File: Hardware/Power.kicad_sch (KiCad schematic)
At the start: 13 parts, among them U22 TLV75733PDRV, U7 SY8205FCC, U9 AP2112K-1.8

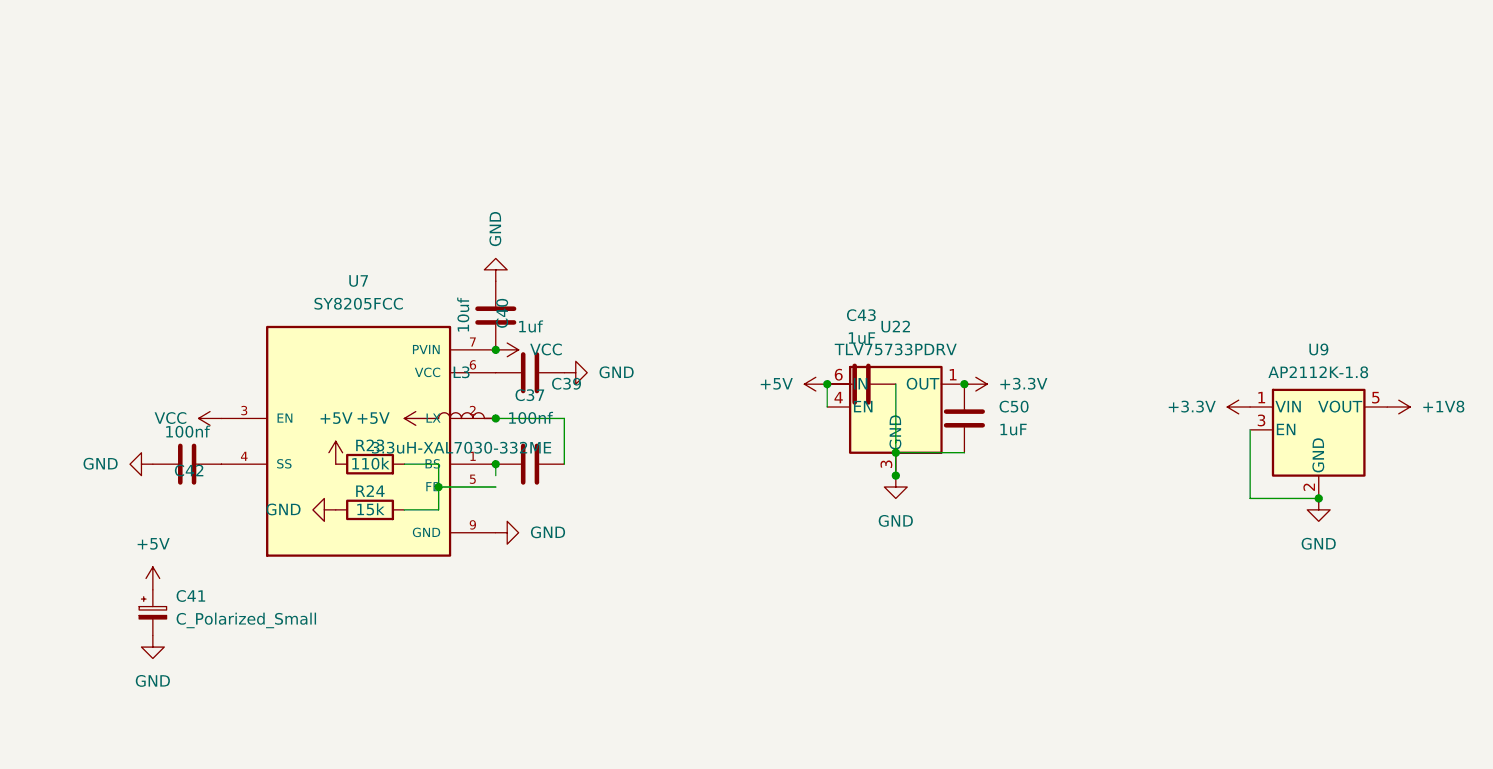
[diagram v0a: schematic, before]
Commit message: 12-March update
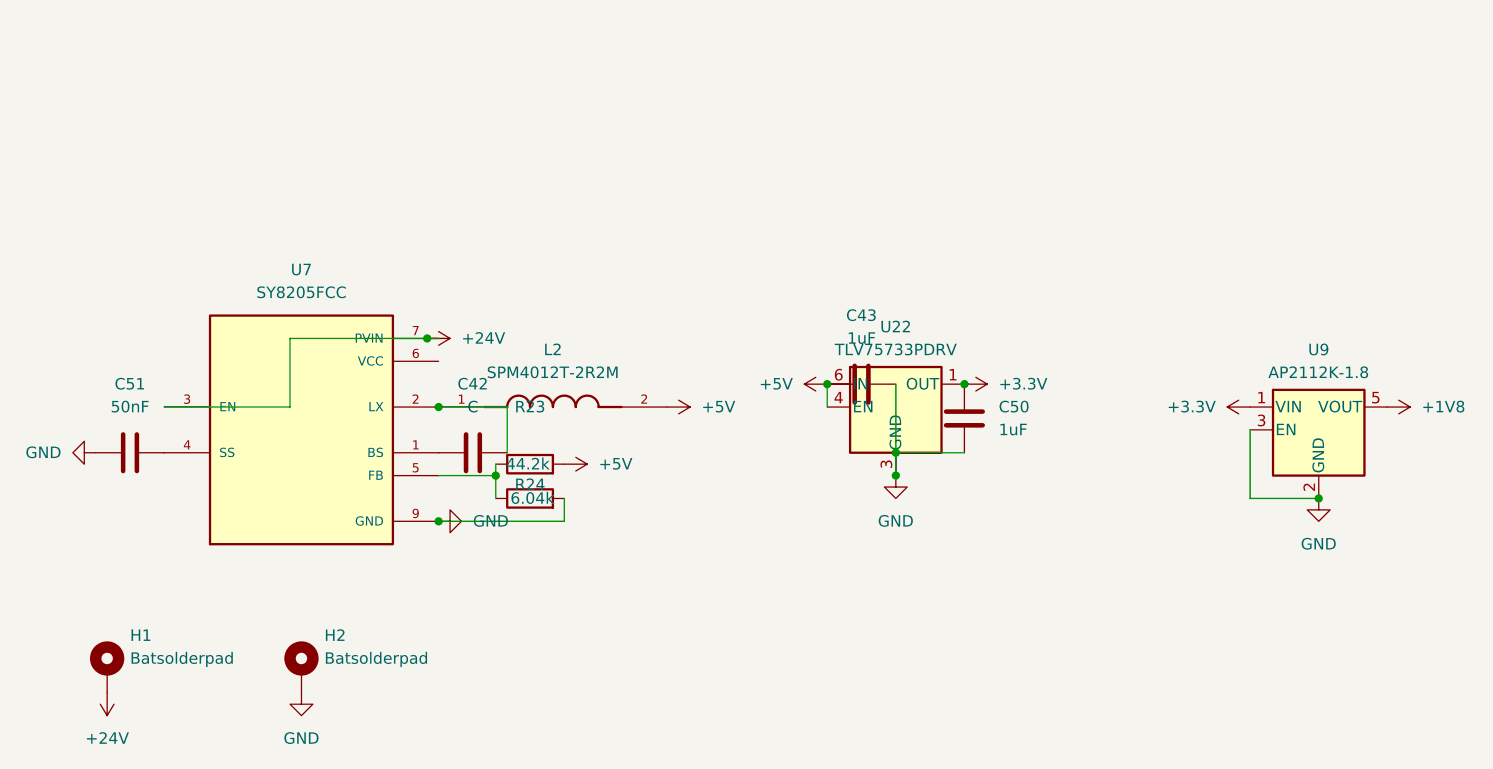
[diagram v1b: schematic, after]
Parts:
- removed C37: 100nf, Capacitor_SMD:C_1206_3216Metric_Pad1.33x1.80mm_HandSolder, symbol Device:C
- removed C39: 1uf, Capacitor_SMD:C_1206_3216Metric_Pad1.33x1.80mm_HandSolder, symbol Device:C
- removed C40: 10uf, Capacitor_SMD:C_0402_1005Metric, symbol Device:C
- removed C41: C_Polarized_Small, Capacitor_SMD:CP_Elec_3x5.3, symbol Device:C_Polarized_Small
- removed L3: 3.3uH-XAL7030-332ME, Inductor_SMD:L_6.3x6.3_H3, symbol Device:L
- added C51: 50nF, Capacitor_SMD:C_0201_0603Metric, symbol Device:C
- added H1, H2: Batsolderpad, TestPoint:TestPoint_Pad_4.0x4.0mm, symbol Mechanical:Batsolderpad
- added L2: SPM4012T-2R2M, SPM4012T-2R2M:IND_SPM4012T-2R2M, symbol SPM4012T-2R2M:SPM4012T-2R2M
- C42: value 100nf -> C; footprint Capacitor_SMD:C_0402_1005Metric -> (none)
- R23: value 110k -> 44.2k; footprint Resistor_SMD:R_0508_1220Metric_Pad1.12x2.15mm_HandSolder -> Resistor_SMD:R_0402_1005Metric
- R24: value 15k -> 6.04k; footprint Resistor_SMD:R_0508_1220Metric -> Resistor_SMD:R_0402_1005Metric
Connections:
- net +5V: now also R23.2, L2.2; no longer R23.1
- net GND: now also R24.2, C51.1, H2.1; no longer C42.1, R24.1
- net at C42.2: now also U7.2 (LX), L2.1; no longer U7.4 (SS)
- net at U7.1 (BS): now also C42.1
- net PVIN renamed +24V
- net +24V: now also H1.1
- new net: R23.1, R24.1, U7.5 (FB)
- new net: C51.2, U7.4 (SS)

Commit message: test gpg
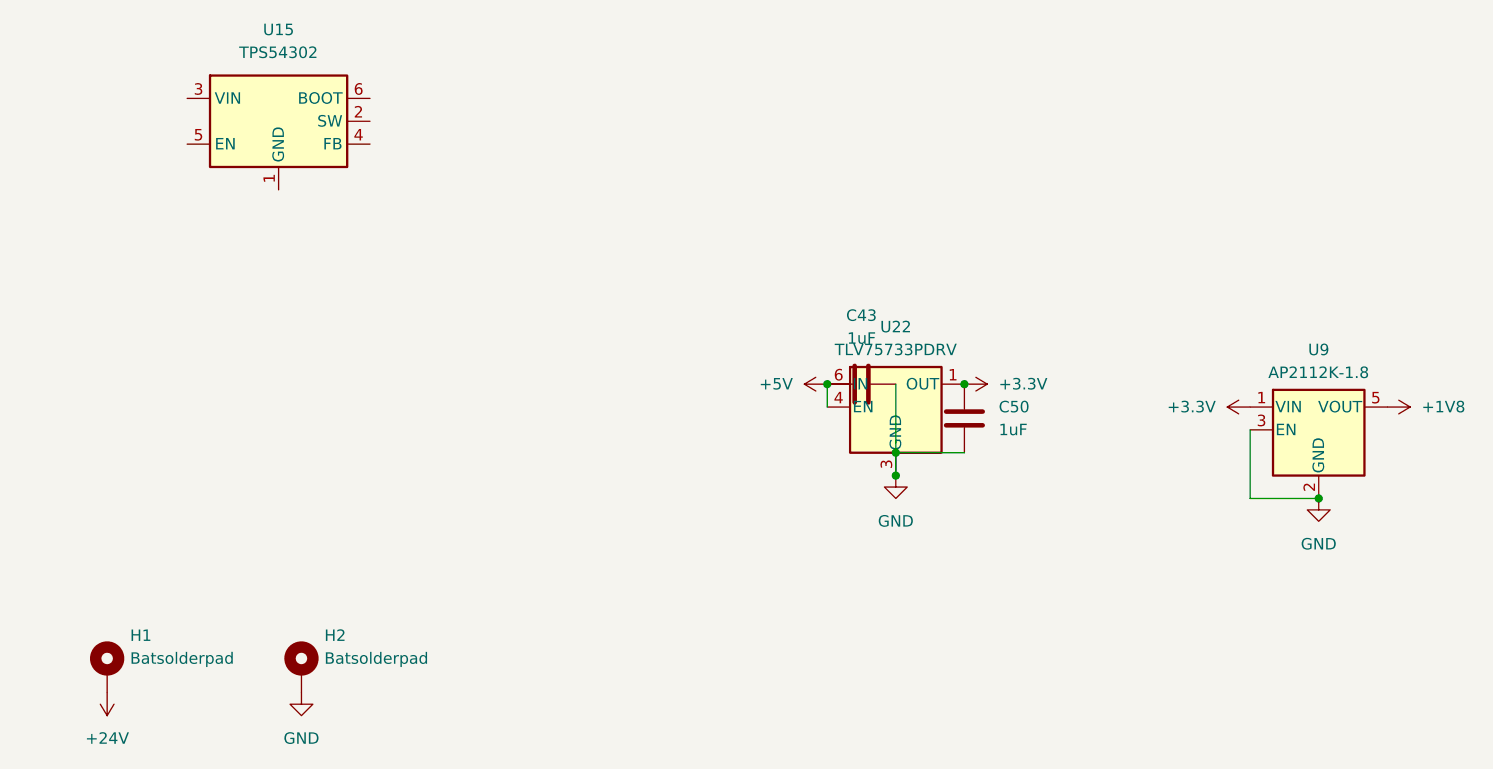
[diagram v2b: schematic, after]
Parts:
- removed C42: C, symbol Device:C
- removed C51: 50nF, Capacitor_SMD:C_0201_0603Metric, symbol Device:C
- removed L2: SPM4012T-2R2M, SPM4012T-2R2M:IND_SPM4012T-2R2M, symbol SPM4012T-2R2M:SPM4012T-2R2M
- removed R23: 44.2k, Resistor_SMD:R_0402_1005Metric, symbol Device:R
- removed R24: 6.04k, Resistor_SMD:R_0402_1005Metric, symbol Device:R
- removed U7: SY8205FCC, SY8205FCC:VREG_SY8205FCC, symbol SY8205FCC:SY8205FCC
- added U15: TPS54302, Package_TO_SOT_SMD:SOT-23-6, symbol Regulator_Switching:TPS54302
